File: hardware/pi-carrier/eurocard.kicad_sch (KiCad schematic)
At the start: 77 parts, among them J1 DIN41612_C96_male_ra_molliebus, J2 Console, J3 Console, J4 Conn_02x20_Odd_Even, J5 Conn_02x20_raspberry_pi4B, J9 Conn_02x05_Odd_Even, U1 74LVC1G07, U10 Lite-on LTP747KR, U11 TCAN332DR, U12 MCP2518FD, U2 TCAN332DR, U3 LM1117IMPX-3.3, U4 74LVC2G04, U5 74LVC2G38, U6 STM32F103C8T6, U8 SN74AHCT125PWR, U9 MAX7219CWG, X1 ASE-40.000MHz-LC, X2 ASE-8.000MHz-LC, Y1 ABS07-32.768KHZ-6-T

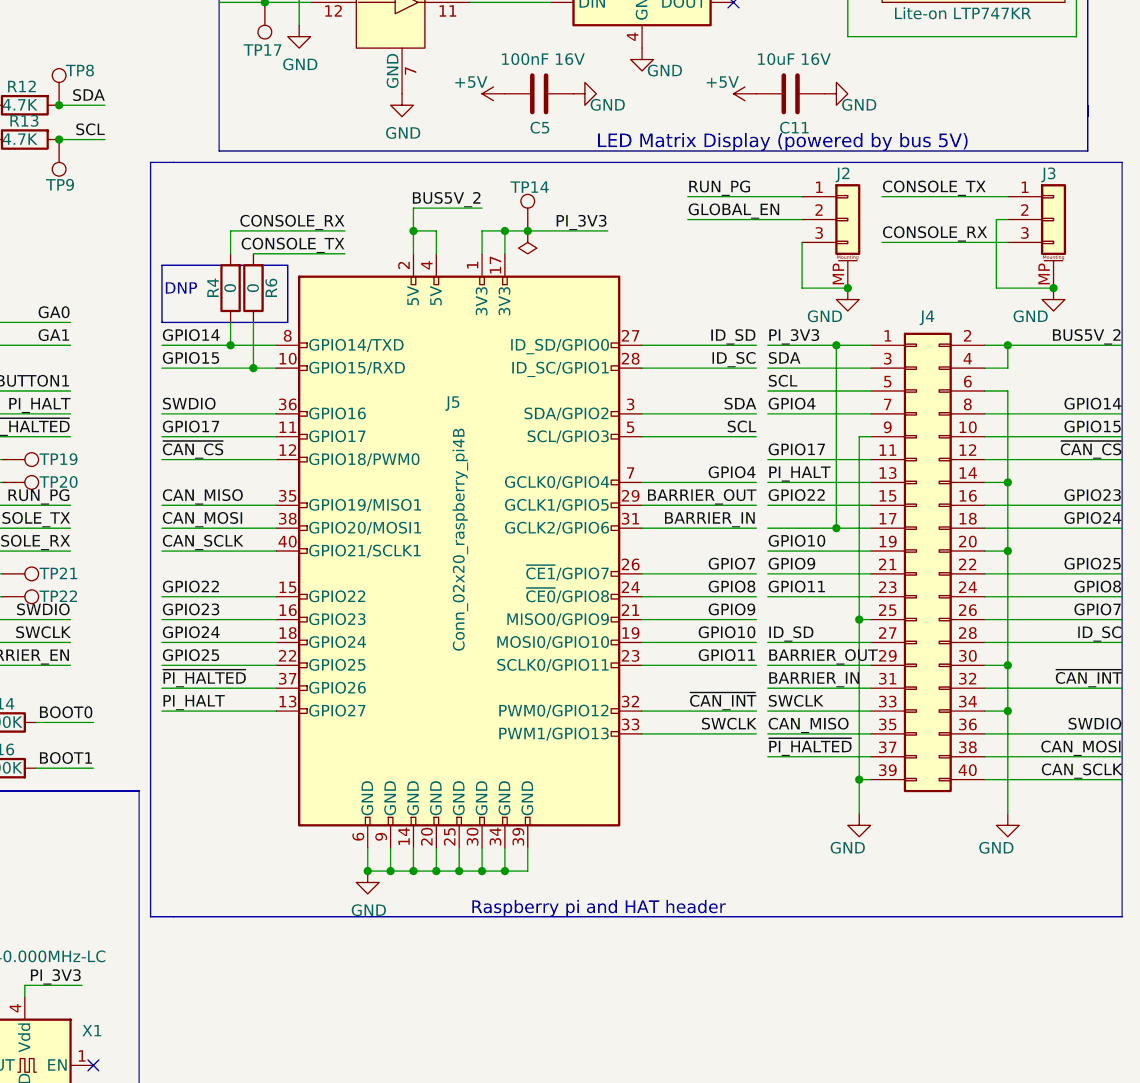
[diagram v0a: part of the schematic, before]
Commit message: pi-carrier: make room for M.2
- remove J4 HAT connector and mounting holes
- relocate components to make space for M.2
- move heartbeat LED and debug J9 near STM32
- drop GPIO console connection, just use JST connector
- reroute traces
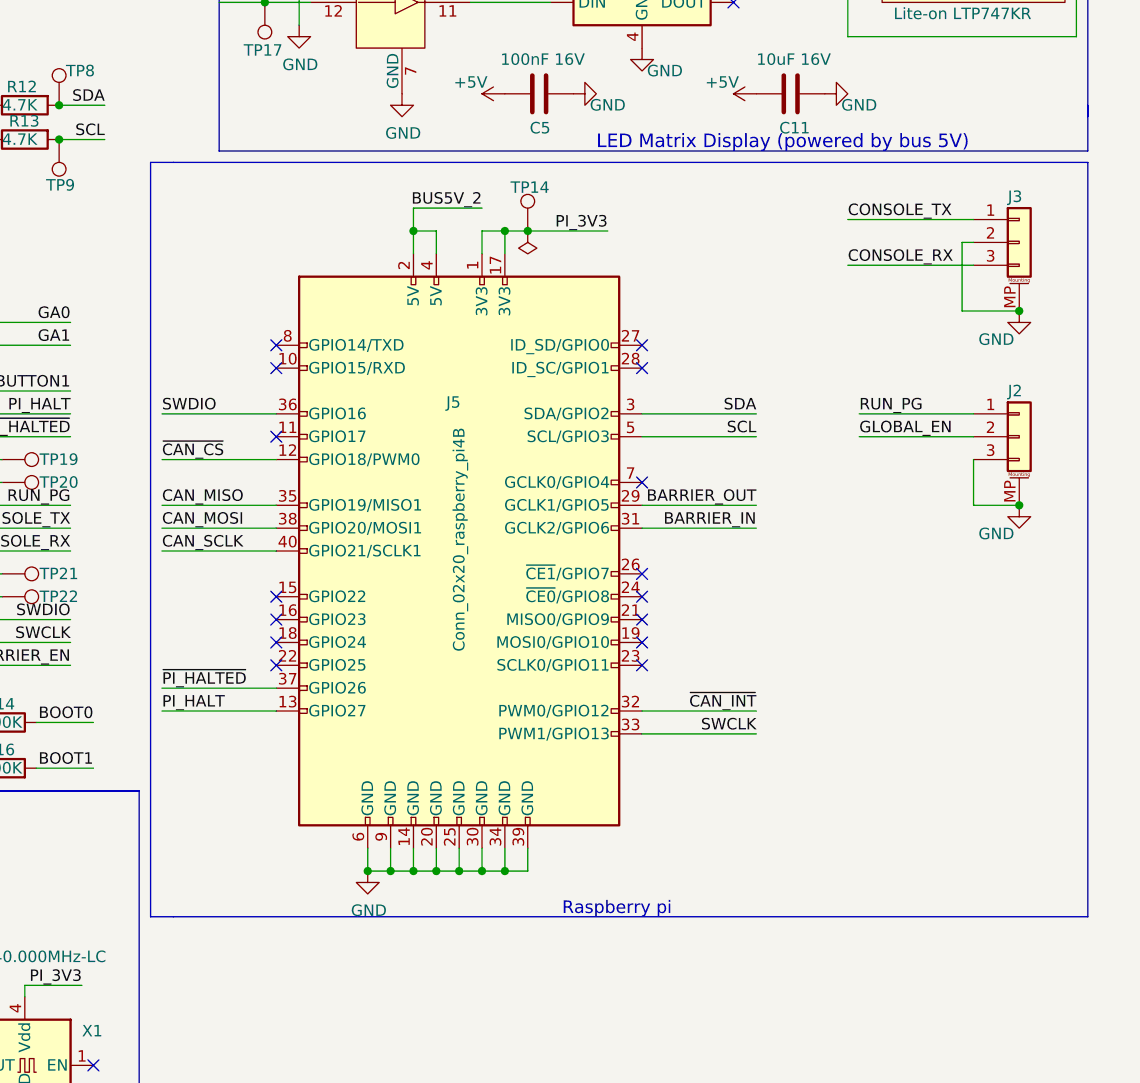
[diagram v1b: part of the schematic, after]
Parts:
- removed J4: Conn_02x20_Odd_Even, 00_eurocard:Rasp_pi_hat_socket, symbol Connector_Generic:Conn_02x20_Odd_Even
- removed R4, R6: 0, Resistor_SMD:R_0603_1608Metric, symbol Device:R
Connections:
- net GPIO10: no longer names the net of J5.19 (MOSI0/GPIO10)
- net GPIO11: no longer names the net of J5.23 (SCLK0/GPIO11)
- net GPIO14: no longer names the net of J5.8 (GPIO14/TXD)
- net GPIO15: no longer names the net of J5.10 (GPIO15/RXD)
- net GPIO17: no longer names the net of J5.11 (GPIO17)
- net GPIO22: no longer names the net of J5.15 (GPIO22)
- net GPIO23: no longer names the net of J5.16 (GPIO23)
- net GPIO24: no longer names the net of J5.18 (GPIO24)
- net GPIO25: no longer names the net of J5.22 (GPIO25)
- net GPIO4: no longer names the net of J5.7 (GCLK0/GPIO4)
- net GPIO7: no longer names the net of J5.26 (~{CE1}/GPIO7)
- net GPIO8: no longer names the net of J5.24 (~{CE0}/GPIO8)
- net GPIO9: no longer names the net of J5.21 (MISO0/GPIO9)
- net ID_SC: no longer names the net of J5.28 (ID_SC/GPIO1)
- net ID_SD: no longer names the net of J5.27 (ID_SD/GPIO0)
- no-connect marks 52 -> 67
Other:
- note added: "Raspberry pi"
- note removed: "DNP"
- note removed: "Raspberry pi and HAT header"
- moved on the sheet: J2, J3
